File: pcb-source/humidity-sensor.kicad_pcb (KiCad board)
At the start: 2 copper layers, 34.2 x 22.6 mm, 71 parts, among them J1 Conn_ARM_JTAG_SWD_10, J2 Conn_02x03_Odd_Even, Q1 Q_NMOS_GSD, Q2 Q_NMOS_GSD, U1 STM32L051C8Tx, U2 SHTC3, U3 SYN115, Y1 13.56MHz, Y2 DNU

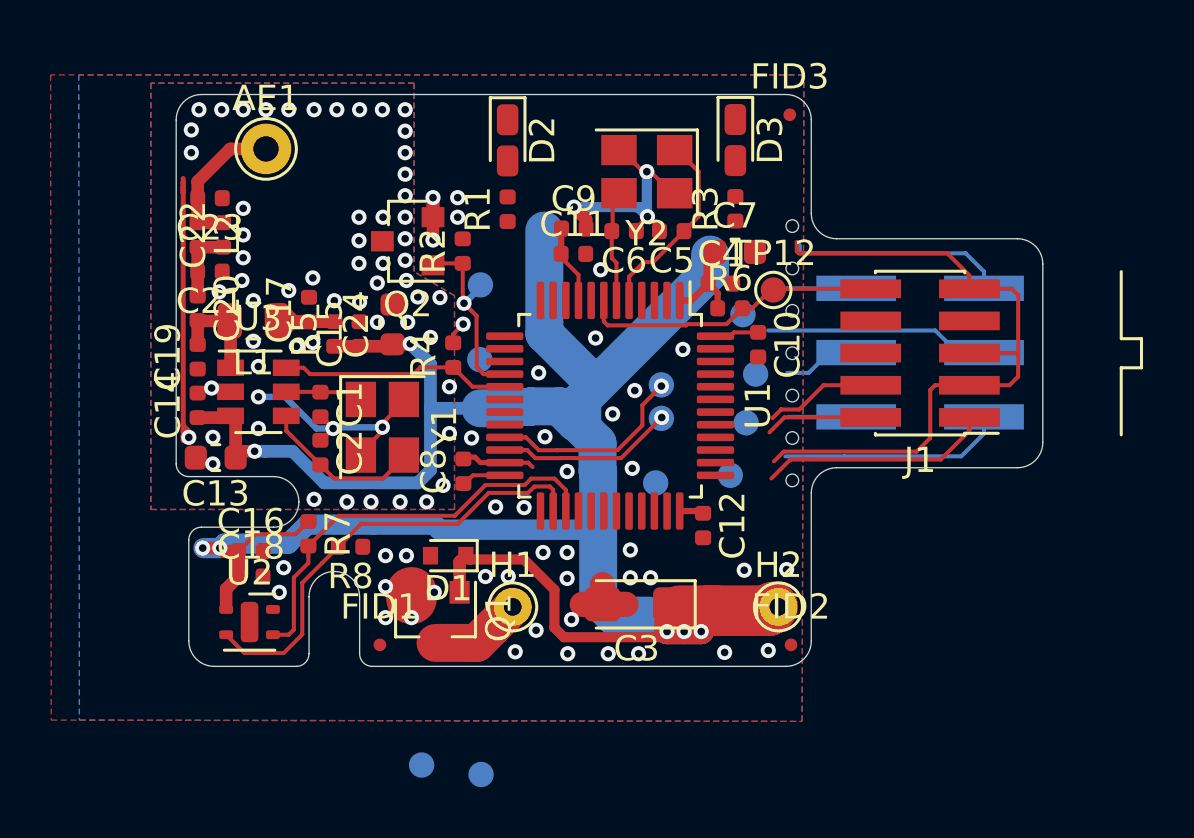
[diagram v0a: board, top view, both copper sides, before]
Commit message: Finish routing
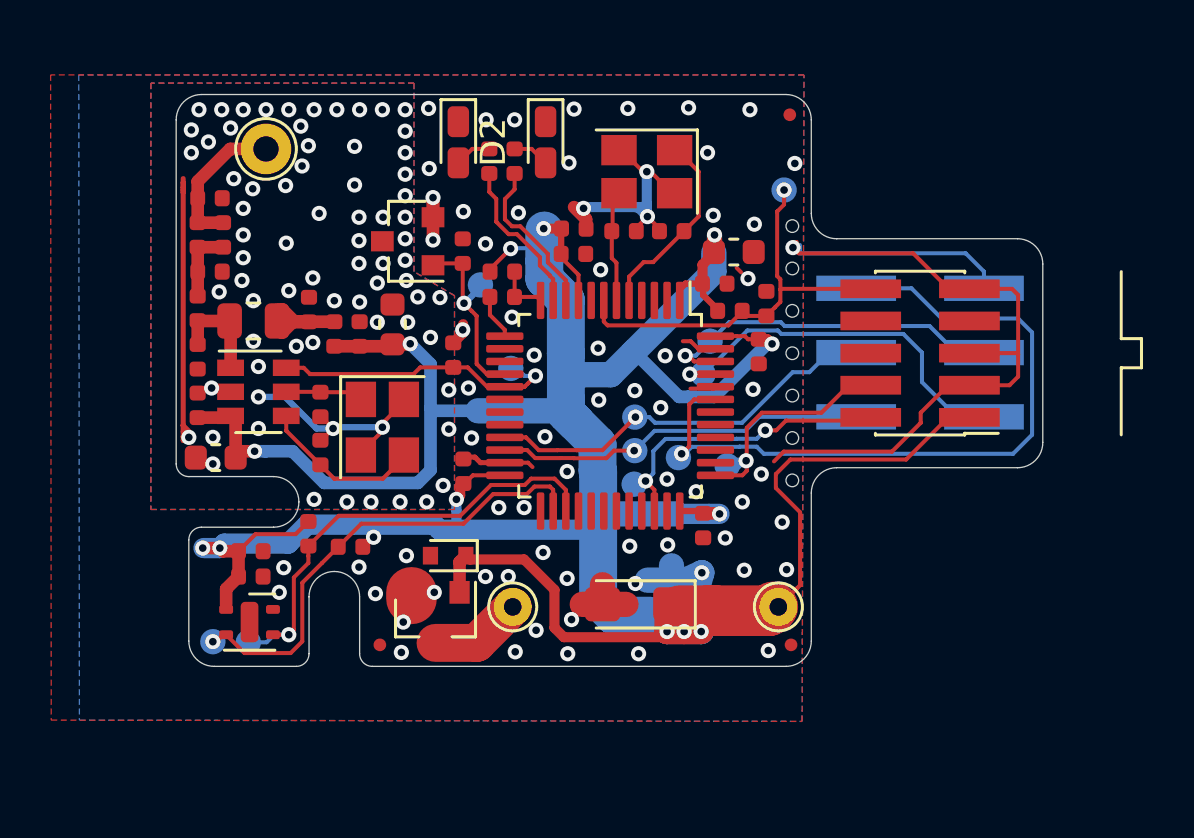
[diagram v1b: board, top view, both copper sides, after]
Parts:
- added C25: 0.1uF, Capacitor_SMD:C_0402_1005Metric, F.Cu at (102.0, 75.5)
- added R10: 100K, Resistor_SMD:R_0402_1005Metric, F.Cu at (91.5, 75.2)
- added R9: 100K, Resistor_SMD:R_0402_1005Metric, F.Cu at (91.5, 74.2)
- added TP13: TP_VCC, TestPoint:TestPoint_Pad_D1.0mm, B.Cu at (97.1, 87.8)
- added TP14: TP_GND, TestPoint:TestPoint_Pad_D1.0mm, B.Cu at (98.2, 86.5)
- TP12: moved to B.Cu
- TP5: value TP_UART_RX -> TP_UART_TX
- TP6: value TP_UART_TX -> TP_UART_RX
- moved TP3 10.6 mm to (81.5, 88.8)
- moved TP4 9.58 mm to (80.1, 88.8)
- moved R3 8.93 mm to (92.0, 69.8)
- moved D3 7.50 mm to (93.2, 69.1)
- moved TP12 3.97 mm to (102.7, 71.0)
- moved TP7 3.01 mm to (98.5, 81.5)
- moved TP6 2.80 mm to (96.8, 81.3), turned to 0 degrees
- moved TP8 2.08 mm to (99.5, 78.2)
- moved R1 2.03 mm to (91.0, 69.8)
- moved D2 1.95 mm to (89.8, 69.1)
- moved TP9 1.67 mm to (99.8, 77.0)
- moved TP2 1.27 mm to (91.9, 78.0)
- moved TP5 1.05 mm to (96.8, 80.0), turned to 0 degrees
- moved TP10 0.85 mm to (96.8, 82.6)
- moved TP11 0.40 mm to (100.4, 81.9)
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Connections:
- J2 pad 1: /UART_TX -> /UART_RX
- J2 pad 3: /UART_RX -> /UART_TX
- TP5 pad 1: /UART_RX -> /UART_TX
- TP6 pad 1: /UART_TX -> /UART_RX
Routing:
- net VCC: track 120.0 -> 150.0 mm, vias 7 -> 14
- net /DEBUG_1: track 3.42 -> 29.5 mm, vias 0 -> 1
- net /SWDIO: track 4.24 -> 12.3 mm, vias 0 -> 2
- net /DEBUG_2: track 8.88 -> 15.8 mm, vias 0 -> 1
- net GND: track 56.4 -> 63.2 mm, vias 46 -> 69
- net Net-(R3-Pad1): track 0.00 -> 6.37 mm
- net Net-(R1-Pad1): track 0.00 -> 6.26 mm
- net /UART_TX: track 10.6 -> 16.6 mm
- net /SWCLK: track 4.42 -> 10.3 mm, vias 0 -> 1
- net Net-(C25-Pad1): track 12.1 -> 17.7 mm, vias 0 -> 1
- net /DEBUG_3: track 8.89 -> 14.2 mm, vias 0 -> 1
- net /UART_RX: track 10.7 -> 14.7 mm
- net /RF_DATA: track 9.09 -> 11.6 mm, vias 0 -> 1
- net Net-(R10-Pad1): track 0.00 -> 2.03 mm
- net Net-(R10-Pad2): track 0.00 -> 1.89 mm
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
